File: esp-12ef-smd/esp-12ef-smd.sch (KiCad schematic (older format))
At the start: 18 parts, among them J1 Battery, J2 USB-TTL, J3 BME280_CONNECTOR, SW1 RESET, U1 ESP-12F

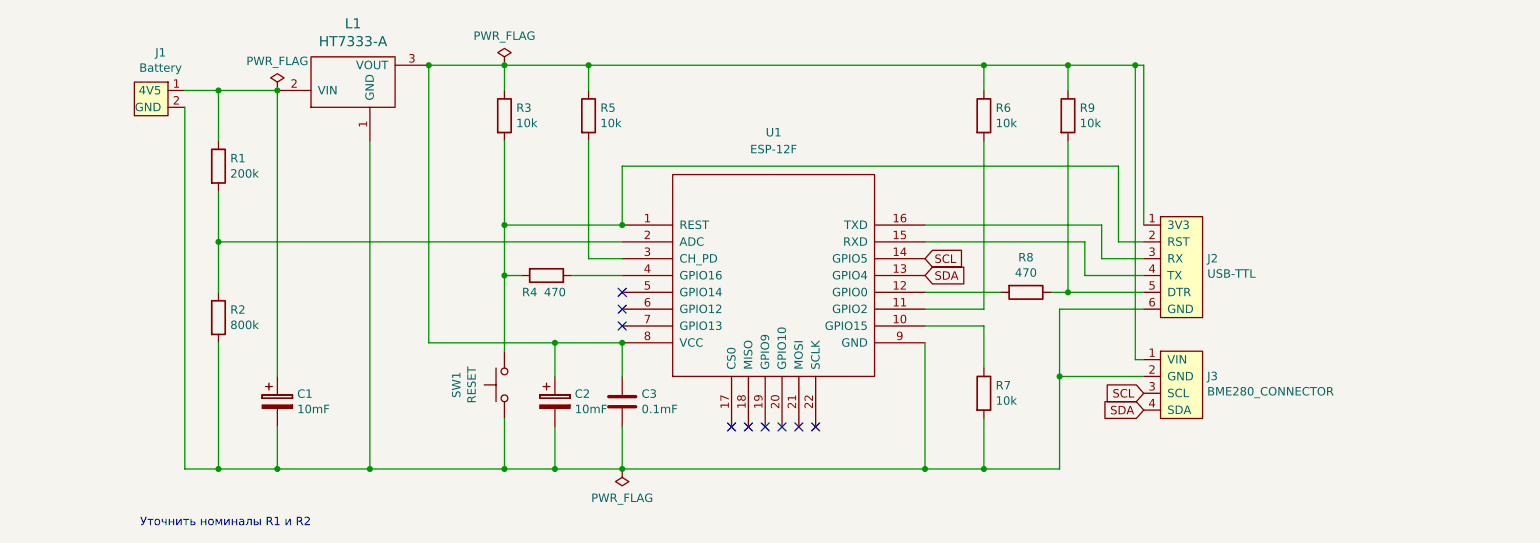
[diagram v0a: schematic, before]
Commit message: minor changes
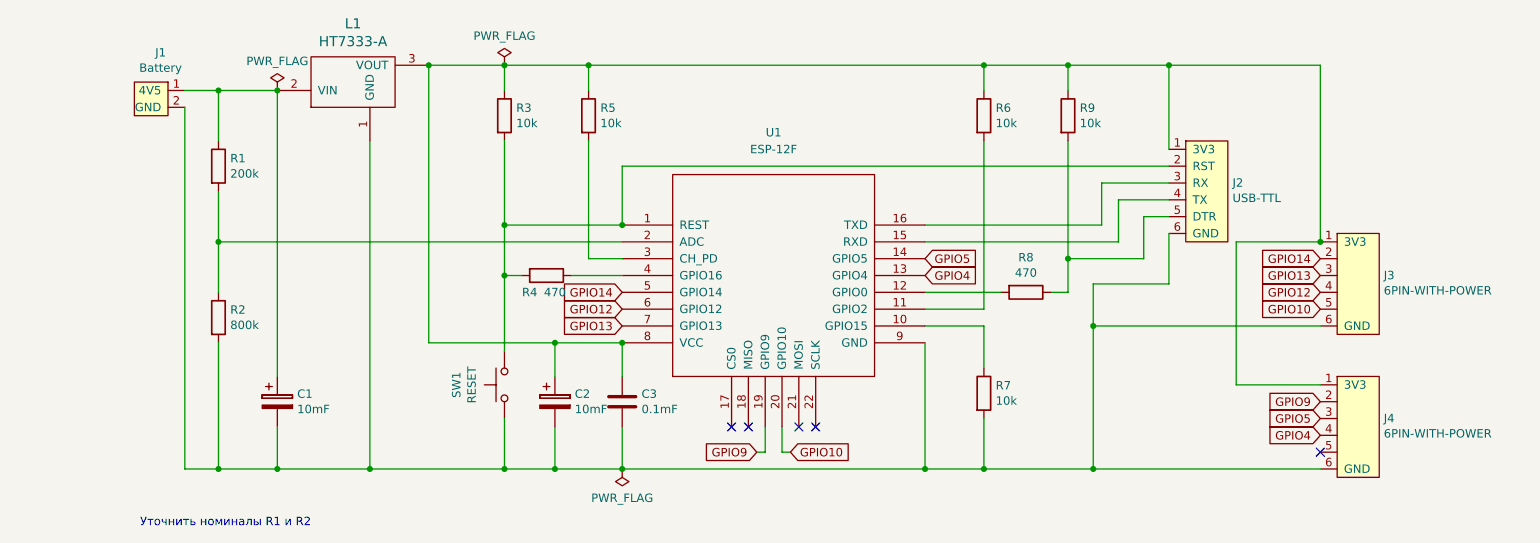
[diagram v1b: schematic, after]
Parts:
- removed J3: BME280_CONNECTOR, Connector_PinSocket_2.54mm:PinSocket_1x04_P2.54mm_Vertical, symbol AlBalLib:BME280_CONNECTOR
- added J3, J4: 6PIN-WITH-POWER, Connector_PinSocket_2.54mm:PinSocket_1x06_P2.54mm_Vertical, symbol AlBalLib:6PIN-WITH-POWER
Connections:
- net GPIO9: now reaches U1.19 (GPIO9)
- net GPIO9: now also J4.2
- net GPIO10: now reaches U1.20 (GPIO10)
- net GPIO10: now also J3.5
- net GPIO14: now reaches U1.5 (GPIO14)
- net GPIO14: now also J3.2
- net GPIO12: now reaches U1.6 (GPIO12)
- net GPIO12: now also J3.4
- net GPIO13: now reaches U1.7 (GPIO13)
- net GPIO13: now also J3.3
- net at C2.1, C3.1, J2.1 (3V3)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: now also J3.1 (3V3), J4.1 (3V3)
- net at C1.2, C2.2, C3.2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: now also J3.6 (GND), J4.6 (GND)
- net SCL renamed GPIO5
- net GPIO5: now also J4.3
- net SDA renamed GPIO4
- net GPIO4: now also J4.4
- no-connect marks 9 -> 5
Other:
- moved on the sheet: J2
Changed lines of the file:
@@
 EESchema Schematic File Version 4
+LIBS:esp-12ef-smd-cache
 EELAYER 26 0
 EELAYER END
@@
 L AlBalLib:USB-TTL J2
 U 1 1 5C5CFE61
-P 7850 3300
-F 0 "J2" H 8228 3051 50  0000 L CNN
-F 1 "USB-TTL" H 8228 2960 50  0000 L CNN
-F 2 "Connector_PinSocket_2.54mm:PinSocket_1x06_P2.54mm_Vertical" H 7850 3300 50  0001 C CNN
-F 3 "" H 7850 3300 50  0001 C CNN
-	1    7850 3300
-	1    0    0    -1
-$EndComp
-Wire Wire Line
-	7850 3350 7850 2400
-Wire Wire Line
-	7850 2400 7800 2400
+P 8000 2850
+F 0 "J2" H 8378 2601 50  0000 L CNN
+F 1 "USB-TTL" H 8378 2510 50  0000 L CNN
+F 2 "Connector_PinSocket_2.54mm:PinSocket_1x06_P2.54mm_Vertical" H 8000 2850 50  0001 C CNN
+F 3 "" H 8000 2850 50  0001 C CNN
+	1    8000 2850
+	1    0    0    -1
+$EndComp
 $Comp
 L Device:R R8
@@
 	7400 2400 6900 2400
 Wire Wire Line
-	7400 2850 7400 3750
-Connection ~ 7400 3750
-Wire Wire Line
-	7400 3750 7850 3750
+	7400 2850 7400 3550
 Wire Wire Line
 	6900 2850 6900 3850
@@
 	6900 2400 4550 2400
 Wire Wire Line
-	6550 3450 7500 3450
-Wire Wire Line
-	7500 3450 7500 3650
-Wire Wire Line
-	7500 3650 7850 3650
-Wire Wire Line
 	6550 3350 7600 3350
-Wire Wire Line
-	7600 3350 7600 3550
-Wire Wire Line
-	7600 3550 7850 3550
 Wire Wire Line
 	4550 2400 4550 2550
@@
 NoConn ~ 5400 4550
 NoConn ~ 5500 4550
-NoConn ~ 5600 4550
-NoConn ~ 5700 4550
 NoConn ~ 5800 4550
 NoConn ~ 5900 4550
-NoConn ~ 4750 3750
-NoConn ~ 4750 3850
-NoConn ~ 4750 3950
 $Comp
 L ht7333-a:HT7333-A L1
@@
 	2150 4800 2350 4800
 Connection ~ 2700 4800
-Wire Wire Line
-	7850 3450 7700 3450
-Wire Wire Line
-	7700 3450 7700 3000
-Wire Wire Line
-	7700 3000 4750 3000
 Wire Wire Line
 	4750 3000 4750 3350
@@
 	-1   0    0    1
 $EndComp
-Wire Wire Line
-	6900 4800 7350 4800
-Wire Wire Line
-	7350 4800 7350 4250
-Wire Wire Line
-	7350 3850 7850 3850
 Connection ~ 6900 4800
-Wire Wire Line
-	7800 2400 7800 4150
-Wire Wire Line
-	7800 4150 7850 4150
-Connection ~ 7800 2400
-Wire Wire Line
-	7800 2400 7400 2400
-Wire Wire Line
-	7850 4250 7350 4250
-Connection ~ 7350 4250
-Wire Wire Line
-	7350 4250 7350 3850
-Text GLabel 6550 3550 2    50   Input ~ 0
-SCL
-Text GLabel 6550 3650 2    50   Input ~ 0
-SDA
-Text GLabel 7850 4350 0    50   Input ~ 0
-SCL
-Text GLabel 7850 4450 0    50   Input ~ 0
-SDA
-$Comp
-L AlBalLib:BME280_CONNECTOR J3
-U 1 1 5C5C841E
-P 7900 4100
-F 0 "J3" H 8227 3951 50  0000 L CNN
-F 1 "BME280_CONNECTOR" H 8227 3860 50  0000 L CNN
-F 2 "Connector_PinSocket_2.54mm:PinSocket_1x04_P2.54mm_Vertical" H 7900 4100 50  0001 C CNN
-F 3 "" H 7900 4100 50  0001 C CNN
-	1    7900 4100
-	1    0    0    -1
-$EndComp
 $Comp
 L Device:R R1
@@
 Wire Wire Line
 	2350 3450 2350 3750
+Text GLabel 4750 3750 0    50   Input ~ 0
+GPIO14
+Text GLabel 4750 3850 0    50   Input ~ 0
+GPIO12
+Text GLabel 4750 3950 0    50   Input ~ 0
+GPIO13
+Text GLabel 6550 3550 2    50   Input ~ 0
+GPIO5
+Text GLabel 6550 3650 2    50   Input ~ 0
+GPIO4
+Text GLabel 5550 4700 0    50   Input ~ 0
+GPIO9
+Text GLabel 5750 4700 2    50   Input ~ 0
+GPIO10
+Wire Wire Line
+	5600 4550 5600 4700
+Wire Wire Line
+	5600 4700 5550 4700
+Wire Wire Line
+	5700 4550 5700 4700
+Wire Wire Line
+	5700 4700 5750 4700
+Wire Wire Line
+	4750 3000 8000 3000
+Wire Wire Line
+	8000 3100 7600 3100
+Wire Wire Line
+	7600 3100 7600 3350
+Wire Wire Line
+	7700 3450 7700 3200
+Wire Wire Line
+	7700 3200 8000 3200
+Wire Wire Line
+	6550 3450 7700 3450
+Wire Wire Line
+	6900 4800 7550 4800
+Wire Wire Line
+	7400 3550 7850 3550
+Wire Wire Line
+	7850 3550 7850 3300
+Wire Wire Line
+	7850 3300 8000 3300
+Connection ~ 7400 3550
+Wire Wire Line
+	7400 3550 7400 3750
+Wire Wire Line
+	8000 2900 8000 2400
+Wire Wire Line
+	7400 2400 8000 2400
+Wire Wire Line
+	8000 3400 8000 3700
+Wire Wire Line
+	8000 3700 7550 3700
+Wire Wire Line
+	7550 3700 7550 3950
+Text GLabel 8900 3550 0    50   Input ~ 0
+GPIO14
+Text GLabel 8900 3750 0    50   Input ~ 0
+GPIO12
+Text GLabel 8900 3650 0    50   Input ~ 0
+GPIO13
+Text GLabel 8900 4400 0    50   Input ~ 0
+GPIO9
+Text GLabel 8900 3850 0    50   Input ~ 0
+GPIO10
+Text GLabel 8900 4500 0    50   Input ~ 0
+GPIO5
+Text GLabel 8900 4600 0    50   Input ~ 0
+GPIO4
+$Comp
+L AlBalLib:6PIN-WITH-POWER J3
+U 1 1 5CA38485
+P 8900 3400
+F 0 "J3" H 9277 3151 50  0000 L CNN
+F 1 "6PIN-WITH-POWER" H 9277 3060 50  0000 L CNN
+F 2 "Connector_PinSocket_2.54mm:PinSocket_1x06_P2.54mm_Vertical" H 8900 3400 50  0001 C CNN
+F 3 "" H 8900 3400 50  0001 C CNN
+	1    8900 3400
+	1    0    0    -1
+$EndComp
+$Comp
+L AlBalLib:6PIN-WITH-POWER J4
+U 1 1 5CA38513
+P 8900 4250
+F 0 "J4" H 9277 4001 50  0000 L CNN
+F 1 "6PIN-WITH-POWER" H 9277 3910 50  0000 L CNN
+F 2 "Connector_PinSocket_2.54mm:PinSocket_1x06_P2.54mm_Vertical" H 8900 4250 50  0001 C CNN
+F 3 "" H 8900 4250 50  0001 C CNN
+	1    8900 4250
+	1    0    0    -1
+$EndComp
+NoConn ~ 8900 4700
+Wire Wire Line
+	8900 4800 7550 4800
+Connection ~ 7550 4800
+Wire Wire Line
+	8900 3950 7550 3950
+Connection ~ 7550 3950
+Wire Wire Line
+	7550 3950 7550 4800
+Wire Wire Line
+	8000 2400 8900 2400
+Connection ~ 8000 2400
+Wire Wire Line
+	8900 2400 8900 3450
+Wire Wire Line
+	8900 3450 8400 3450
+Wire Wire Line
+	8400 3450 8400 4300
+Wire Wire Line
+	8400 4300 8900 4300
+Connection ~ 8900 3450
 $EndSCHEMATC
